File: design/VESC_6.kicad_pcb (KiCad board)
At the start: 4 copper layers, 60 x 60 mm, 303 parts, among them P1 USB_OTG, P10 PH_C, P11 SUPPLY, P12 GND, P2 BATT_-, P2 CAN, P4 HALL_ENC, P5 COM, P6 SERVO, P7 SWD, P8 PH_A, P9 PH_B, Q1 IRF7749, Q2 IRF7749, Q3 IRF7749, Q4 IRF7749, Q5 IRF7749, Q6 IRF7749, U1 STM32F40X_LQFP64, U10 MPU9150, U11 SENSOR_VOLTAGE, U2 LM3671, U3 DRV8301, U4 TJA1051TK3, U5 AD8418, U6 AD8418, U7 AD8418, U8 NRF24L01P, U9 CONN_U_FL, X1 8m, X2 16M

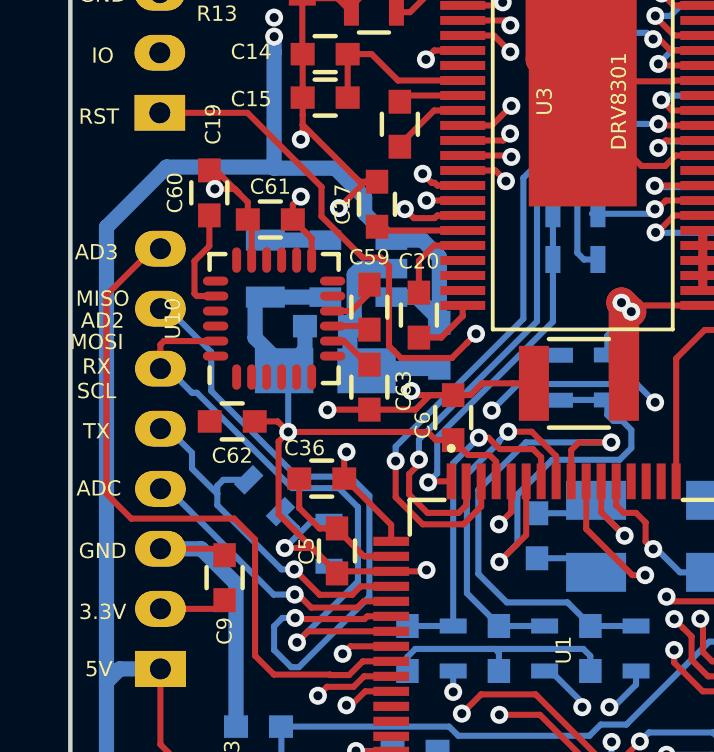
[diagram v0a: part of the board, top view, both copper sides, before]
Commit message: initial commit
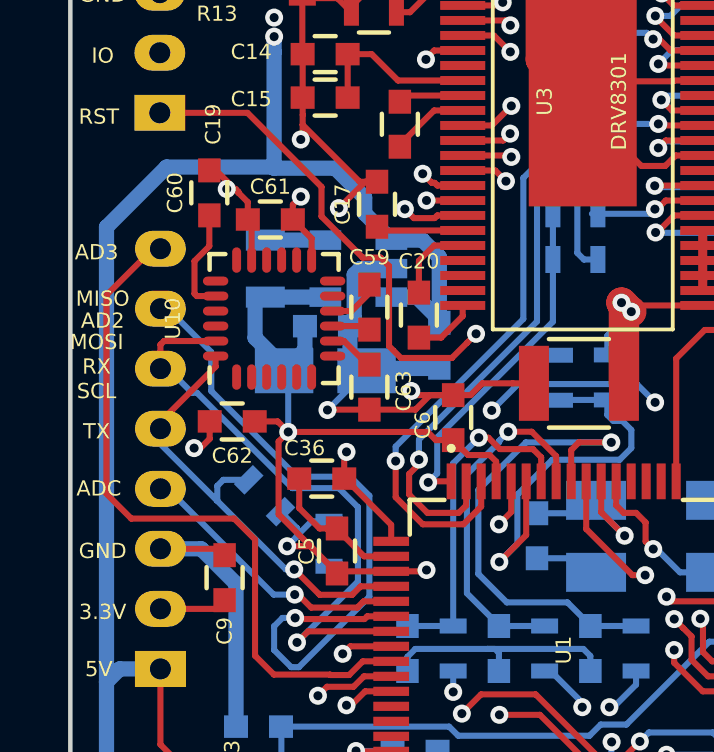
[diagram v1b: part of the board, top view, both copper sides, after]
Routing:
- net /MCU/RX_SDA_NSS: track 12.0 -> 15.2 mm
- net GND: track 204.8 -> 207.5 mm, vias 157 -> 158
